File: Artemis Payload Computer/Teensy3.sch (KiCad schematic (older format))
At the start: 1 part, among them U201 Teensy3.2

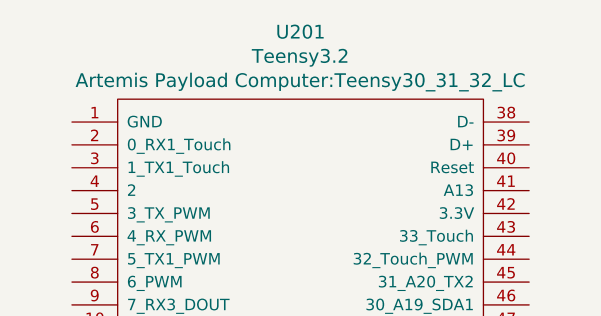
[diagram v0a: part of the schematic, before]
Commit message: I think I undid this...
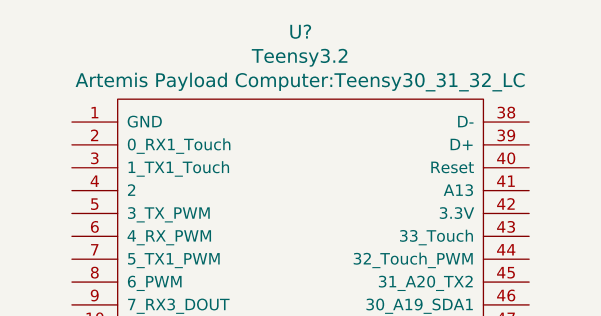
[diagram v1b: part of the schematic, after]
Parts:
- renumbered U201 to U?
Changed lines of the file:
@@
 $Descr A4 11693 8268
 encoding utf-8
-Sheet 2 5
+Sheet 2 4
 Title ""
 Date ""
@@
 $EndDescr
 $Comp
-L Artemis_Footprints:Teensy3.2 U201
+L Artemis_Footprints:Teensy3.2 U?
 U 1 1 6028516C
 P 6350 3600
-F 0 "U201" H 6350 5343 60  0000 C CNN
+F 0 "U?" H 6350 5343 60  0000 C CNN
 F 1 "Teensy3.2" H 6350 5237 60  0000 C CNN
 F 2 "Artemis Payload Computer:Teensy30_31_32_LC" H 6350 5131 60  0000 C CNN

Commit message: Fuck it we're starting over. Sorry for the mess Nathan
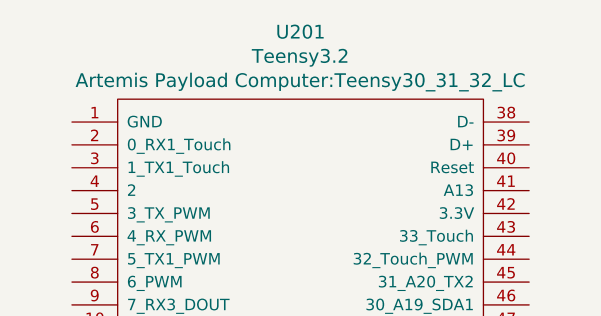
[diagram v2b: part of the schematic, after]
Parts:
- gave numbers to parts that had none: 1
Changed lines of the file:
@@
 $Descr A4 11693 8268
 encoding utf-8
-Sheet 2 4
+Sheet 2 5
 Title ""
 Date ""
@@
 $EndDescr
 $Comp
-L Artemis_Footprints:Teensy3.2 U?
+L Artemis_Footprints:Teensy3.2 U201
 U 1 1 6028516C
 P 6350 3600
-F 0 "U?" H 6350 5343 60  0000 C CNN
+F 0 "U201" H 6350 5343 60  0000 C CNN
 F 1 "Teensy3.2" H 6350 5237 60  0000 C CNN
 F 2 "Artemis Payload Computer:Teensy30_31_32_LC" H 6350 5131 60  0000 C CNN
